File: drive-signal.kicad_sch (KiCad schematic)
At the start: 25 parts, among them J1 Conn_01x03_Pin, J10 Conn_01x04_Pin, J11 Conn_01x04_Pin, J2 Conn_01x03_Pin, J3 Conn_01x03_Pin, J4 Conn_01x03_Pin, J5 Conn_01x03_Pin, J6 Conn_01x03_Pin, J7 Conn_01x02_Pin, J8 Conn_01x04_Pin, J9 Conn_01x04_Pin, U1 STM32F4

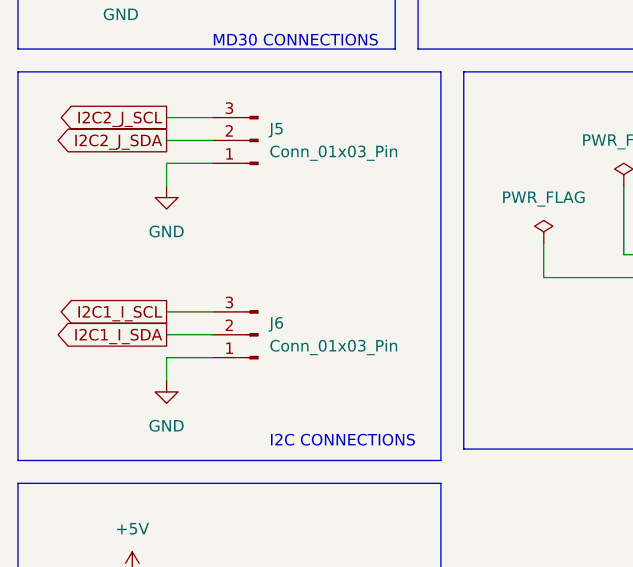
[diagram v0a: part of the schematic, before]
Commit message: incorporate feedback
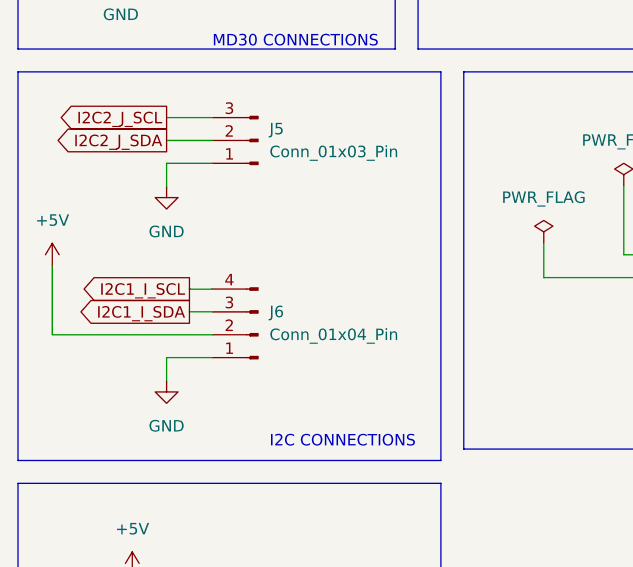
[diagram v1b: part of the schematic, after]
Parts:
- J6: value Conn_01x03_Pin -> Conn_01x04_Pin; footprint Connector_JST:JST_PH_B3B-PH-K_1x03_P2.00mm_Vertical -> Connector_JST:JST_PH_B4B-PH-K_1x04_P2.00mm_Vertical; symbol Connector:Conn_01x03_Pin -> Connector:Conn_01x04_Pin
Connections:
- net +5V: now also J6.2 (Pin_2)
- net I2C1_I_SCL: now also J6.4 (Pin_4); no longer J6.3 (Pin_3)
- net I2C1_I_SDA: now also J6.3 (Pin_3); no longer J6.2 (Pin_2)
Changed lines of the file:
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@@
+    (stroke (width 0) (type default))
+  )
+  (wire (pts (xy 17.78 128.27) (xy 35.56 128.27))
     (stroke (width 0) (type default))
   )
@@
     (stroke (width 0) (type default))
   )
+  (wire (pts (xy 17.78 120.65) (xy 17.78 128.27))
+    (stroke (width 0) (type default))
+  )
   (wire (pts (xy 30.48 43.18) (xy 25.4 43.18))
     (stroke (width 0) (type default))
@@
     (stroke (width 0) (type default))
   )
-  (wire (pts (xy 30.48 128.27) (xy 35.56 128.27))
-    (stroke (width 0) (type default))
-  )
   (wire (pts (xy 26.67 160.02) (xy 26.67 166.37))
     (stroke (width 0) (type default))
@@
     (stroke (width 0) (type default))
   )
+  (wire (pts (xy 33.02 123.19) (xy 35.56 123.19))
+    (stroke (width 0) (type default))
+  )
   (wire (pts (xy 74.93 33.02) (xy 80.01 33.02))
     (stroke (width 0) (type default))
   )
+  (wire (pts (xy 33.02 125.73) (xy 35.56 125.73))
+    (stroke (width 0) (type default))
+  )
   (wire (pts (xy 30.48 106.68) (xy 35.56 106.68))
     (stroke (width 0) (type default))
@@
   )
   (wire (pts (xy 26.67 60.96) (xy 30.48 60.96))
-    (stroke (width 0) (type default))
-  )
-  (wire (pts (xy 30.48 125.73) (xy 35.56 125.73))
     (stroke (width 0) (type default))
   )
@@
     )
   )
-  (global_label "I2C1_I_SDA" (shape output) (at 30.48 128.27 180) (fields_autoplaced)
-    (effects (font (size 1.27 1.27)) (justify right))
-    (property "Intersheetrefs" "${INTERSHEET_REFS}" (at 17.0929 128.27 0)
+  (global_label "I2C1_I_SDA" (shape output) (at 33.02 125.73 180) (fields_autoplaced)
+    (effects (font (size 1.27 1.27)) (justify right))
+    (property "Intersheetrefs" "${INTERSHEET_REFS}" (at 19.6329 125.73 0)
       (effects (font (size 1.27 1.27)) (justify right) hide)
     )
@@
     )
   )
-  (global_label "I2C1_I_SCL" (shape output) (at 30.48 125.73 180) (fields_autoplaced)
-    (effects (font (size 1.27 1.27)) (justify right))
-    (property "Intersheetrefs" "${INTERSHEET_REFS}" (at 17.1534 125.73 0)
+  (global_label "I2C1_I_SCL" (shape output) (at 33.02 123.19 180) (fields_autoplaced)
+    (effects (font (size 1.27 1.27)) (justify right))
+    (property "Intersheetrefs" "${INTERSHEET_REFS}" (at 19.6934 123.19 0)
       (effects (font (size 1.27 1.27)) (justify right) hide)
     )
@@
     )
   )
-  (symbol (lib_id "Connector:Conn_01x03_Pin") (at 40.64 128.27 180) (unit 1)
-    (in_bom yes) (on_board yes) (dnp no) (fields_autoplaced)
-    (property "Reference" "J6" (at 41.91 127 0)
-      (effects (font (size 1.27 1.27)) (justify right))
-    )
-    (property "Value" "Conn_01x03_Pin" (at 41.91 129.54 0)
-      (effects (font (size 1.27 1.27)) (justify right))
-    )
-    (property "Footprint" "Connector_JST:JST_PH_B3B-PH-K_1x03_P2.00mm_Vertical" (at 40.64 128.27 0)
+  (symbol (lib_id "Connector:Conn_01x04_Pin") (at 40.64 128.27 180) (unit 1)
+    (in_bom yes) (on_board yes) (dnp no) (fields_autoplaced)
+    (property "Reference" "J6" (at 41.91 125.73 0)
+      (effects (font (size 1.27 1.27)) (justify right))
+    )
+    (property "Value" "Conn_01x04_Pin" (at 41.91 128.27 0)
+      (effects (font (size 1.27 1.27)) (justify right))
+    )
+    (property "Footprint" "Connector_JST:JST_PH_B4B-PH-K_1x04_P2.00mm_Vertical" (at 40.64 128.27 0)
       (effects (font (size 1.27 1.27)) hide)
     )
@@
     (pin "1")
     (pin "3")
+    (pin "4")
     (instances
       (project "drive-signal"
@@
         )
       )
+    )
+  )
+  (symbol (lib_id "power:+5V") (at 17.78 120.65 0) (unit 1)
+    (in_bom yes) (on_board yes) (dnp no) (fields_autoplaced)
+    (property "Reference" "#PWR025" (at 17.78 124.46 0)
+      (effects (font (size 1.27 1.27)) hide)
+    )
+    (property "Value" "+5V" (at 17.78 115.57 0)
+      (effects (font (size 1.27 1.27)))
+    )
+    (property "Footprint" "" (at 17.78 120.65 0)
+      (effects (font (size 1.27 1.27)) hide)
+    )
+    (property "Datasheet" "" (at 17.78 120.65 0)
+      (effects (font (size 1.27 1.27)) hide)
+    )
+    (pin "1")
+    (instances
+      (project "drive-signal"
+        (path "/0fd5a227-32c1-4fb8-b9b0-22b52f16b2f2"
+          (reference "#PWR025") (unit 1)
+        )
+      )
